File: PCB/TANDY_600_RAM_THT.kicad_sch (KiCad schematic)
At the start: 5 parts, among them J1 DIN 41612 2x22 male right-ang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, U1 628128, U2 74HC08

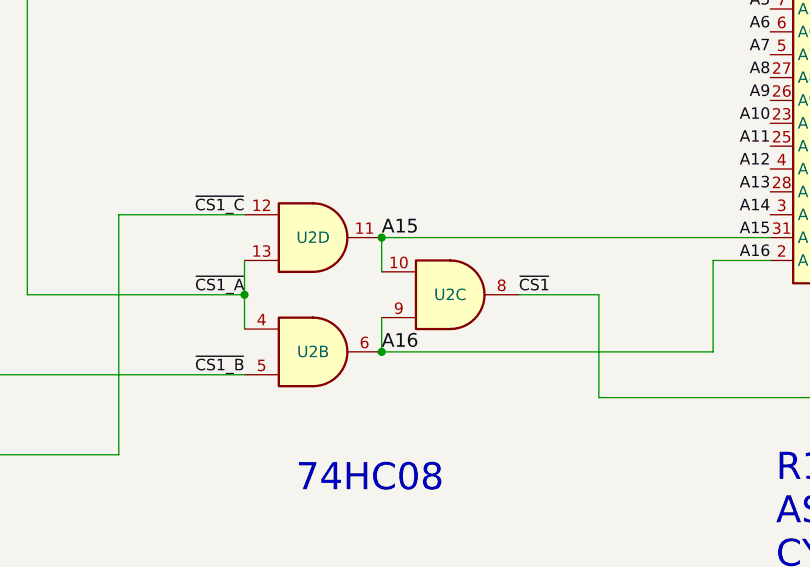
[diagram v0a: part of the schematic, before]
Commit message: dual_008
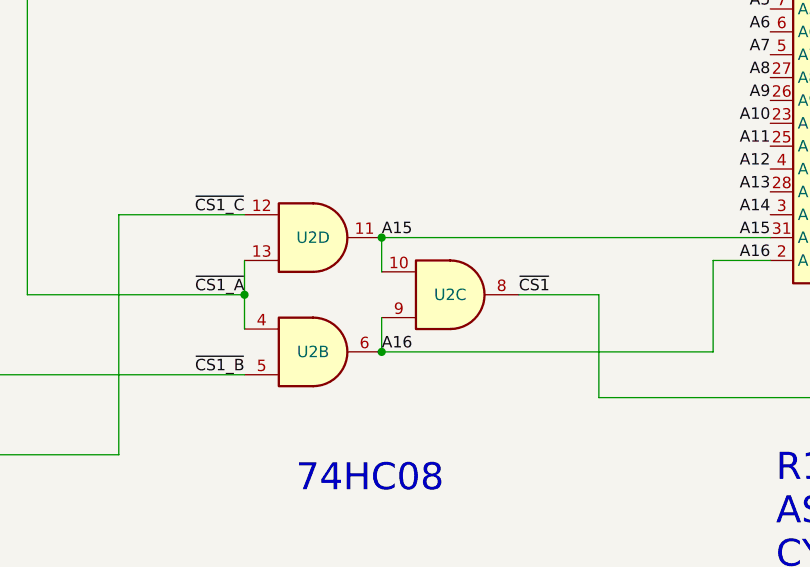
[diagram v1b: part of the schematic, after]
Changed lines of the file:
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@@
   )
   (label "A16" (at 140.97 109.22 0)
-    (effects (font (size 1.524 1.524)) (justify left bottom))
+    (effects (font (size 1.27 1.27)) (justify left bottom))
   )
   (label "A14" (at 66.04 58.42 180)
@@
   )
   (label "A15" (at 140.97 96.52 0)
-    (effects (font (size 1.524 1.524)) (justify left bottom))
+    (effects (font (size 1.27 1.27)) (justify left bottom))
   )
   (label "D3" (at 209.55 66.04 0)
